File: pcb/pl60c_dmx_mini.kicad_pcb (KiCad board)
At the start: 4 copper layers, 38.5 x 28 mm, 37 parts, among them J1 USB-C 16P, J2 XLR-5 female (DMX OUT), Q1 S8050, SW2 BOOT, SW3 USER, U1 ESP32-S3-MINI-1-N8, U2 AP2112K-3.3, U3 SP3485EN, U4 USBLC6-2SC6

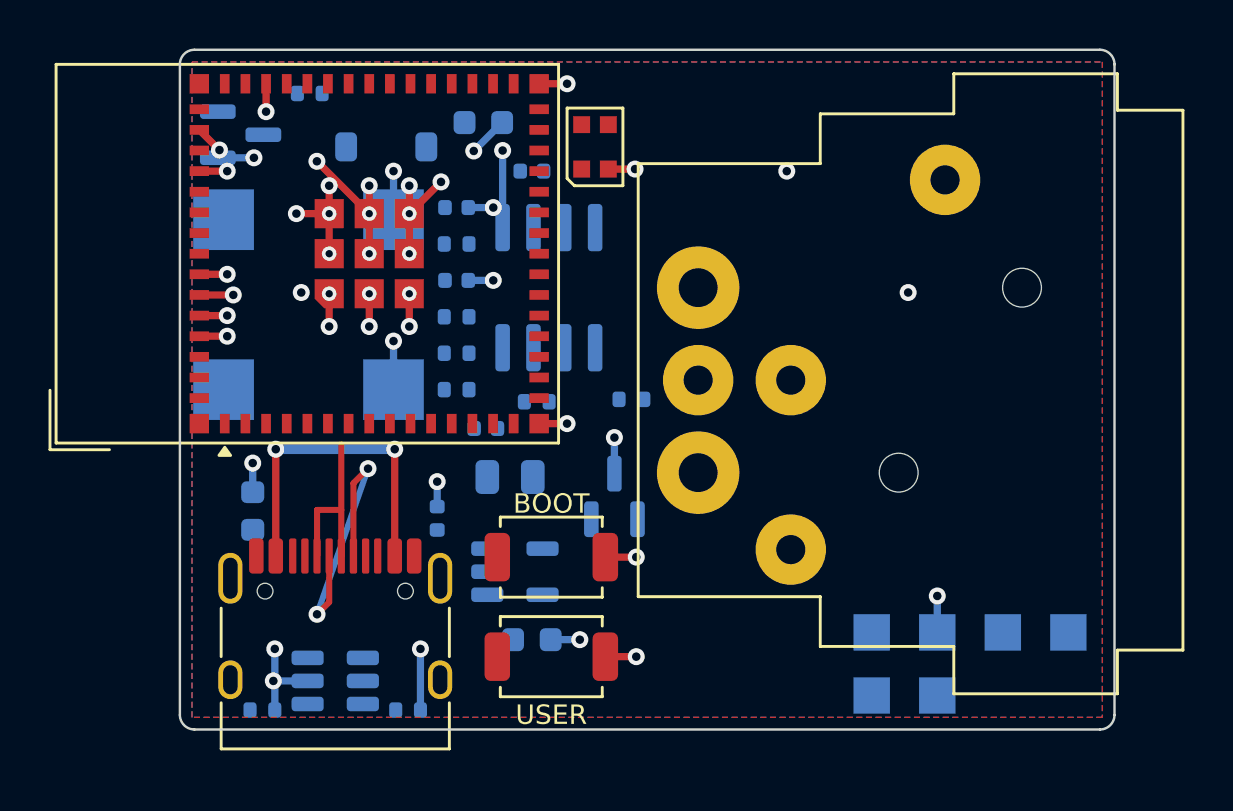
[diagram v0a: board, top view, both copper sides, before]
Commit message: auto: 2026-09-02 13:56:20
Co-Authored-By: Claude Fable 5.1 <noreply@anthropic.com>
Claude-Session: https://claude.ai/code/session_01WsrVZb94LwbHVAmBvsSTfn
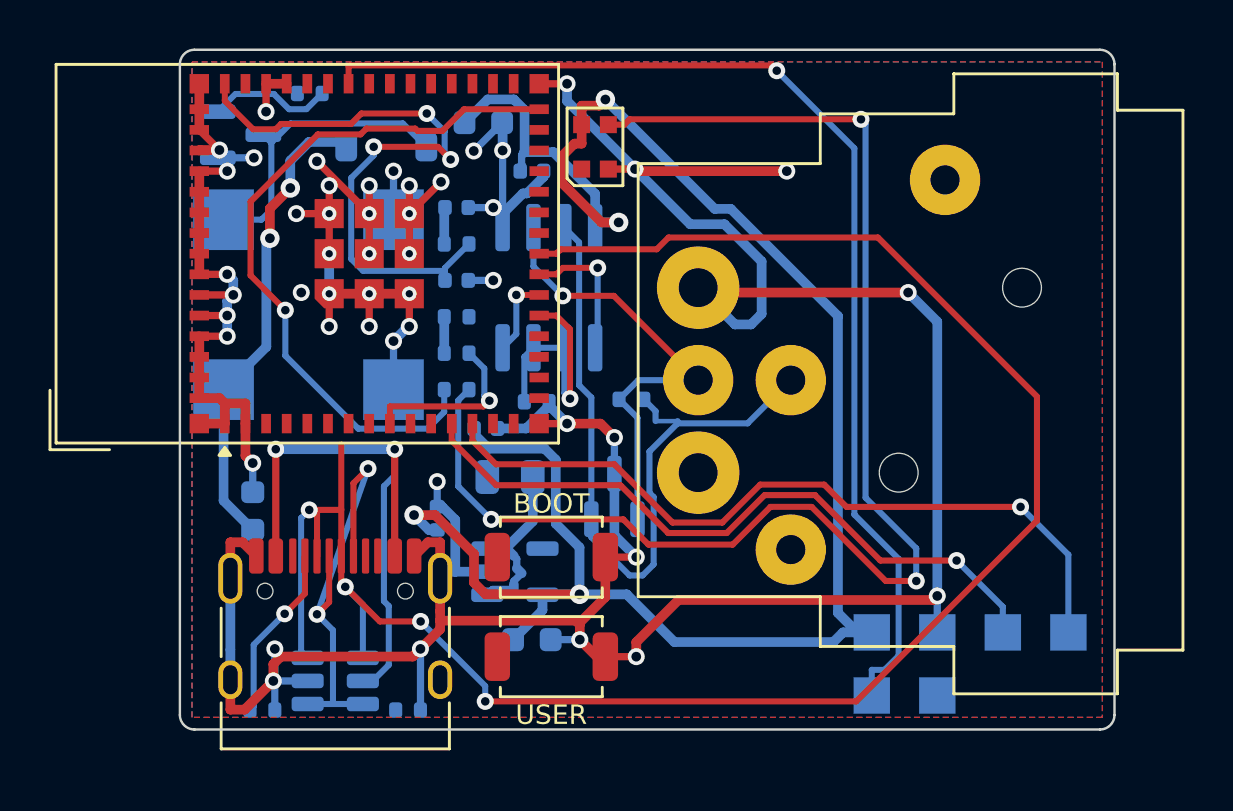
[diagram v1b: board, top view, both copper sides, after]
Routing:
- net GND: track 58.2 -> 196.9 mm
- net +3V3: track 0.00 -> 86.0 mm, vias 0 -> 4
- net USB_D-: track 7.50 -> 81.2 mm, vias 0 -> 4
- net LED_DATA_R: track 0.00 -> 56.4 mm, vias 0 -> 3
- net TXD0: track 0.00 -> 47.0 mm, vias 0 -> 1
- net EXP_SCL: track 0.00 -> 31.7 mm, vias 0 -> 1
- net DMX_B: track 0.00 -> 30.5 mm
- net LED_DATA: track 0.00 -> 29.5 mm, vias 0 -> 1
- net EXP_SDA: track 0.00 -> 28.6 mm, vias 0 -> 1
- net +5V: track 0.00 -> 27.0 mm, vias 0 -> 2
- net EN: track 0.00 -> 26.4 mm, vias 0 -> 3
- net DMX_A: track 0.00 -> 19.2 mm, vias 0 -> 1
- net BZ_N: track 0.00 -> 12.5 mm
- net VBUS: track 13.7 -> 24.2 mm
- net DMX_DE: track 0.00 -> 10.2 mm, vias 0 -> 1
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
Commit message: auto: 2026-09-02 13:58:22
Co-Authored-By: Claude Fable 5.1 <noreply@anthropic.com>
Claude-Session: https://claude.ai/code/session_01WsrVZb94LwbHVAmBvsSTfn
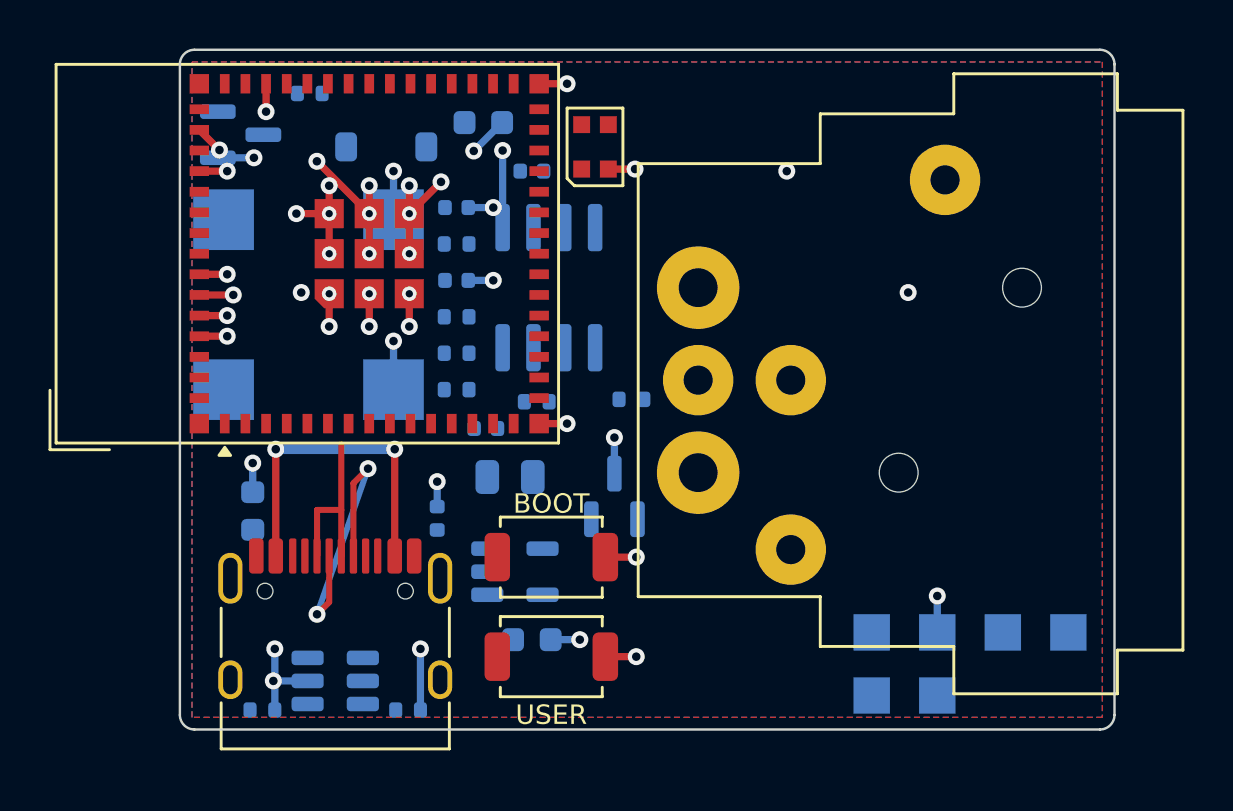
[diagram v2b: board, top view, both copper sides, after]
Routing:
- net GND: track 196.9 -> 58.2 mm
- net +3V3: track 86.0 -> 0.00 mm, vias 4 -> 0
- net USB_D-: track 81.2 -> 7.50 mm, vias 4 -> 0
- net LED_DATA_R: track 56.4 -> 0.00 mm, vias 3 -> 0
- net TXD0: track 47.0 -> 0.00 mm, vias 1 -> 0
- net EXP_SCL: track 31.7 -> 0.00 mm, vias 1 -> 0
- net DMX_B: track 30.5 -> 0.00 mm
- net LED_DATA: track 29.5 -> 0.00 mm, vias 1 -> 0
- net EXP_SDA: track 28.6 -> 0.00 mm, vias 1 -> 0
- net +5V: track 27.0 -> 0.00 mm, vias 2 -> 0
- net EN: track 26.4 -> 0.00 mm, vias 3 -> 0
- net DMX_A: track 19.2 -> 0.00 mm, vias 1 -> 0
- net BZ_N: track 12.5 -> 0.00 mm
- net VBUS: track 24.2 -> 13.7 mm
- net DMX_DE: track 10.2 -> 0.00 mm, vias 1 -> 0
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
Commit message: auto: 2026-09-02 14:00:24
Co-Authored-By: Claude Fable 5.1 <noreply@anthropic.com>
Claude-Session: https://claude.ai/code/session_01WsrVZb94LwbHVAmBvsSTfn
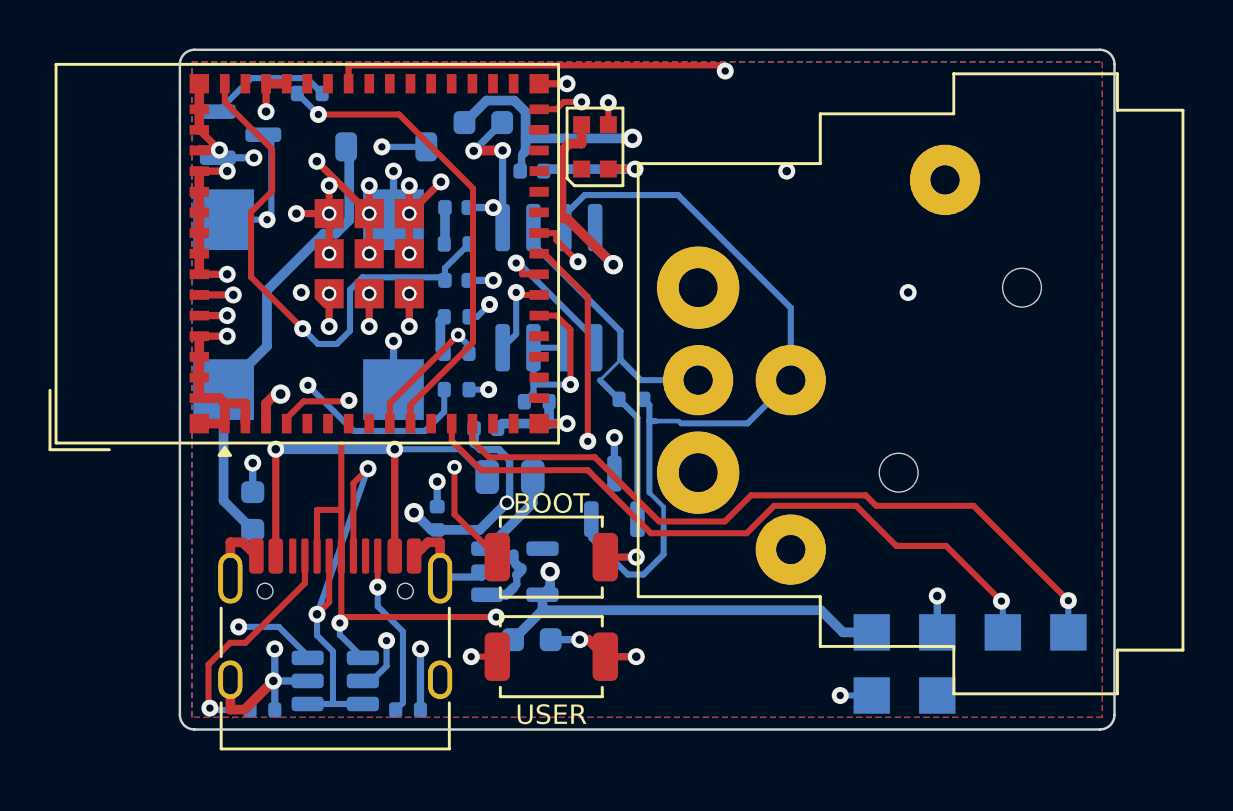
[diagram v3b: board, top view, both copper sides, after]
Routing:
- net GND: track 58.2 -> 166.4 mm
- net +3V3: track 0.00 -> 78.7 mm, vias 0 -> 6
- net TXD0: track 0.00 -> 45.5 mm, vias 0 -> 2
- net USB_D-: track 7.50 -> 45.6 mm, vias 0 -> 4
- net DMX_B: track 0.00 -> 33.1 mm
- net EXP_SCL: track 0.00 -> 30.2 mm, vias 0 -> 1
- net LED_DATA: track 0.00 -> 30.1 mm, vias 0 -> 2
- net USB_D+: track 12.8 -> 41.9 mm, vias 2 -> 3
- net EXP_SDA: track 0.00 -> 28.3 mm, vias 0 -> 1
- net +5V: track 0.00 -> 26.6 mm
- net EN: track 0.00 -> 22.3 mm, vias 0 -> 1
- net IO0_BOOT: track 0.00 -> 20.3 mm, vias 0 -> 3
- net BTN_USER: track 0.00 -> 20.3 mm, vias 0 -> 2
- net BUZZER: track 0.00 -> 19.6 mm, vias 0 -> 1
- net DMX_A: track 0.00 -> 18.0 mm
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
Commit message: auto: 2026-09-02 14:02:26
Co-Authored-By: Claude Fable 5.1 <noreply@anthropic.com>
Claude-Session: https://claude.ai/code/session_01WsrVZb94LwbHVAmBvsSTfn
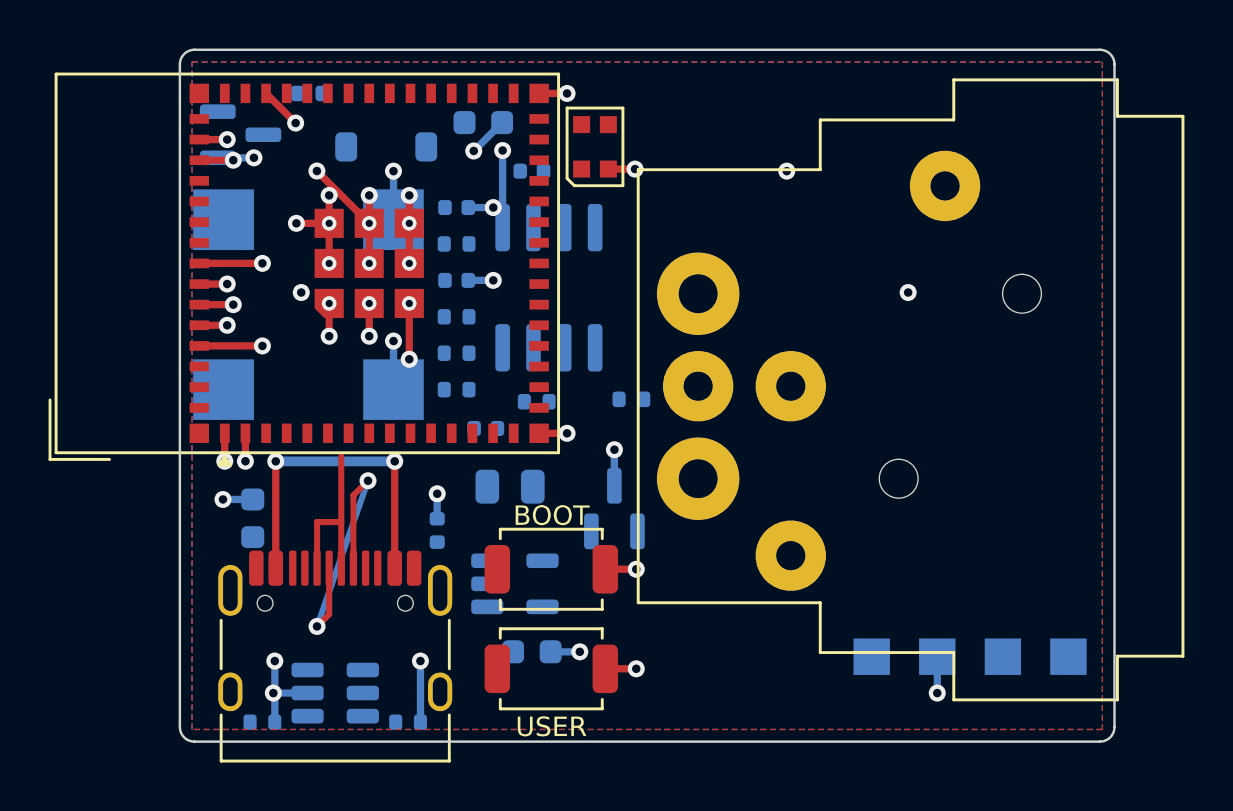
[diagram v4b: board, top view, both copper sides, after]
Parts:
- removed TP5: TXD0, TestPoint_Pad_1.5x1.5mm
- removed TP6: RXD0, TestPoint_Pad_1.5x1.5mm
- moved TP1 1.00 mm to (28.5, 25.0)
- moved TP2 1.00 mm to (31.2, 25.0)
- moved TP3 1.00 mm to (33.9, 25.0)
- moved TP4 1.00 mm to (36.6, 25.0)
- moved C2 0.50 mm to (14.5, 24.8)
- moved C3 0.50 mm to (10.6, 19.8)
- moved D1 0.50 mm to (17.9, 18.9)
- moved J1 0.50 mm to (6.40, 25.4)
- moved R1 0.50 mm to (3.40, 27.7)
- moved R2 0.50 mm to (9.40, 27.7)
- moved SW2 0.50 mm to (15.3, 21.4)
- moved SW3 0.50 mm to (15.3, 25.5)
- moved U2 0.50 mm to (13.8, 22.0)
- moved U4 0.50 mm to (6.40, 26.5)
- moved U1 0.40 mm to (5.25, 8.80)
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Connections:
- U1 pad 39: TXD0 -> (no net)
- U1 pad 40: RXD0 -> (no net)
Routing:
- net GND: track 166.4 -> 64.5 mm, vias 48 -> 50
- net +3V3: track 78.7 -> 0.00 mm, vias 6 -> 0
- net TXD0: track 45.5 -> 0.00 mm, vias 2 -> 0
- net USB_D-: track 45.6 -> 7.50 mm, vias 4 -> 0
- net DMX_B: track 33.1 -> 0.00 mm
- net EXP_SCL: track 30.2 -> 0.00 mm, vias 1 -> 0
- net LED_DATA: track 30.1 -> 0.00 mm, vias 2 -> 0
- net USB_D+: track 41.9 -> 12.8 mm, vias 3 -> 2
- net EXP_SDA: track 28.3 -> 0.00 mm, vias 1 -> 0
- net +5V: track 26.6 -> 0.00 mm
- net EN: track 22.3 -> 0.00 mm, vias 1 -> 0
- net IO0_BOOT: track 20.3 -> 0.00 mm, vias 3 -> 0
- net BTN_USER: track 20.3 -> 0.00 mm, vias 2 -> 0
- net BUZZER: track 19.6 -> 0.00 mm, vias 1 -> 0
- net DMX_A: track 18.0 -> 0.00 mm
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- added copper zone on In2.Cu, net +3V3
- removed copper zone on In2.Cu, net GND
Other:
- board size 38.5 x 28 mm -> 38.5 x 28.5 mm
- board text removed: "TX0 RX0"
